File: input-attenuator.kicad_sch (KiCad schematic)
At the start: 44 parts, among them J1 DC_INTF, J2 RF_IN, J3 RX_1_RF, J4 RX_2_RF, K1 EE2-5TNU-L, K2 EE2-5TNU-L, K3 EE2-5TNU-L, K4 EE2-5TNU-L, Q1 MMBT3904, Q2 MMBT3904, Q3 MMBT3904, Q4 MMBT3904, Q5 MMBT3904, Q6 MMBT3904, Q7 MMBT3904, Q8 MMBT3904, U1 74HC595

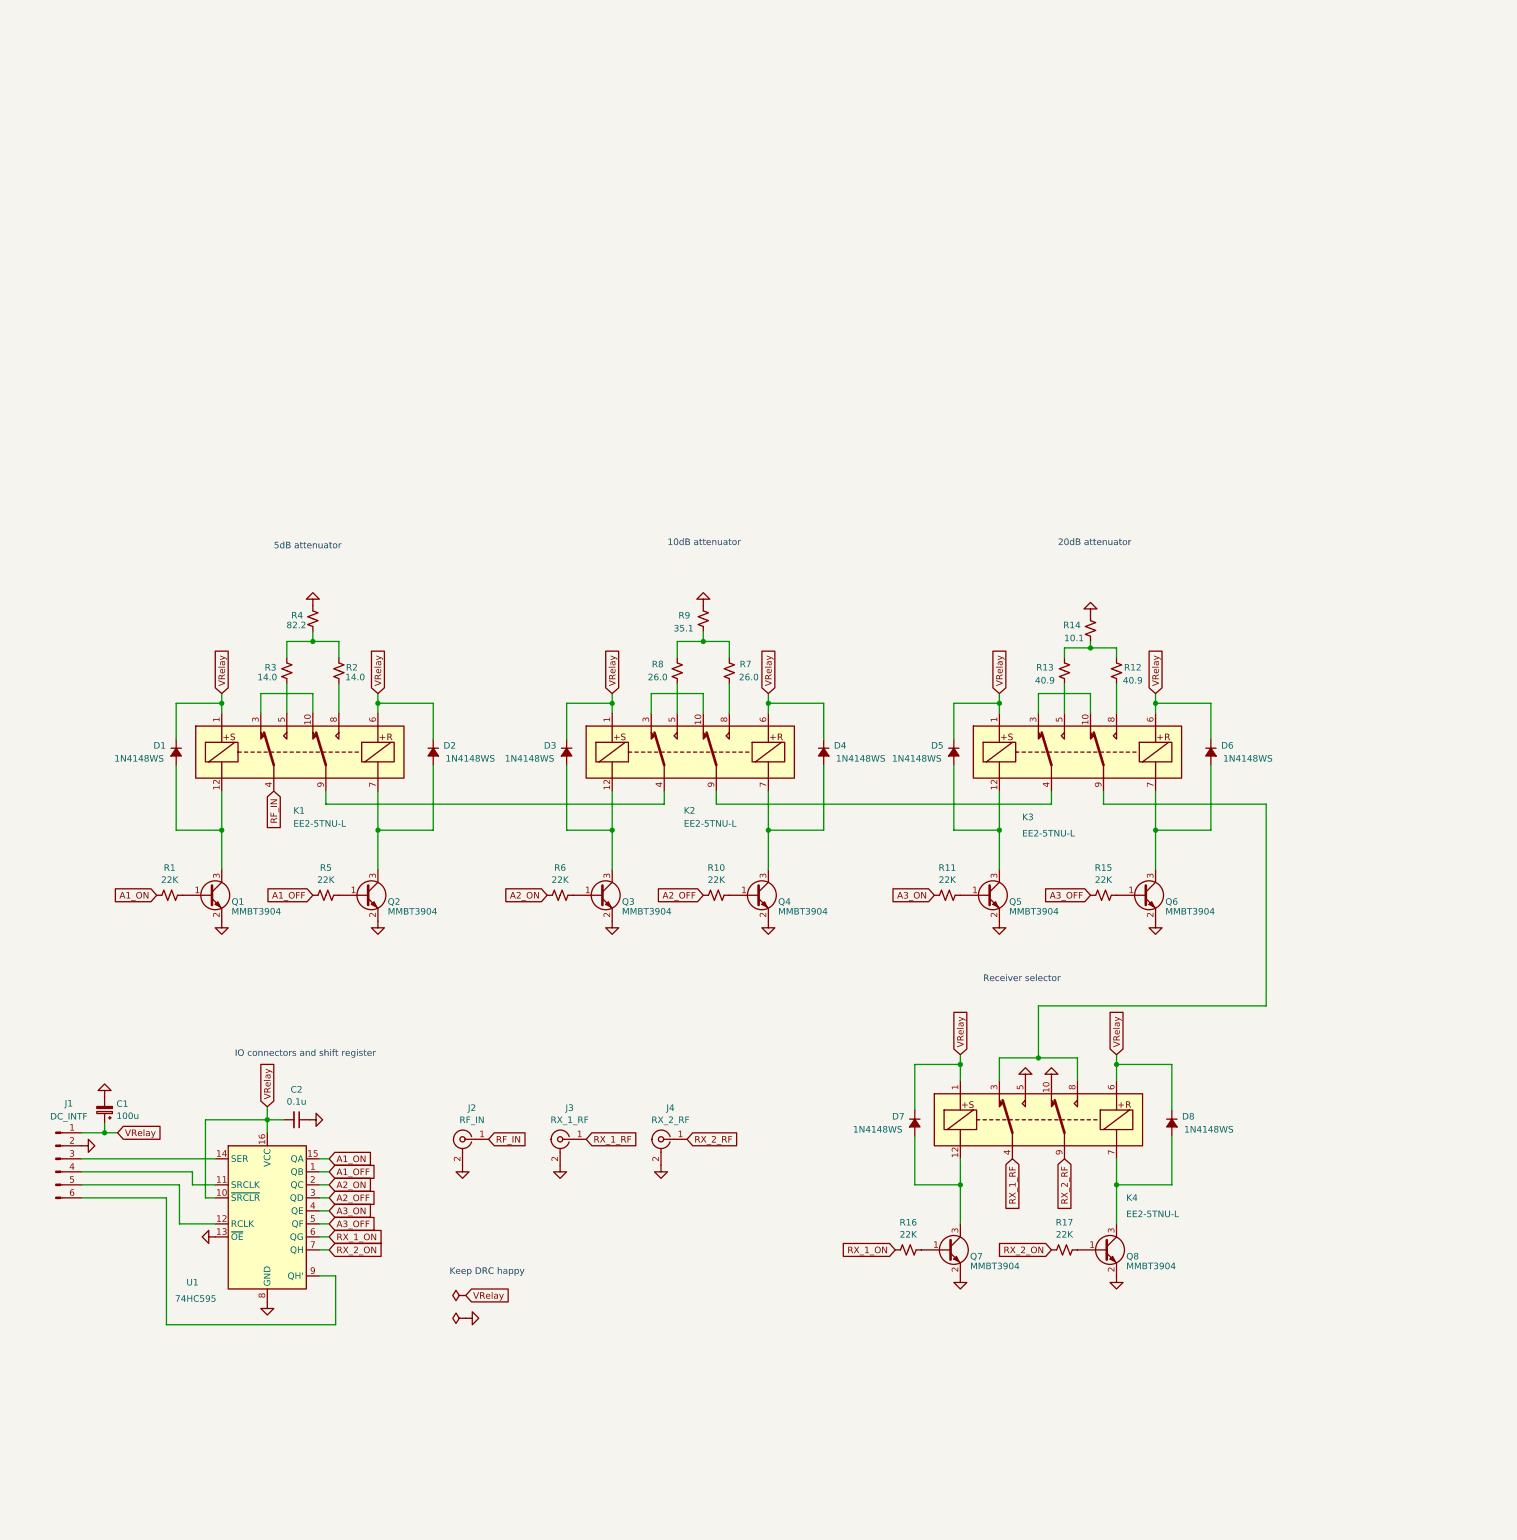
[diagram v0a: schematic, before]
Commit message: noComment
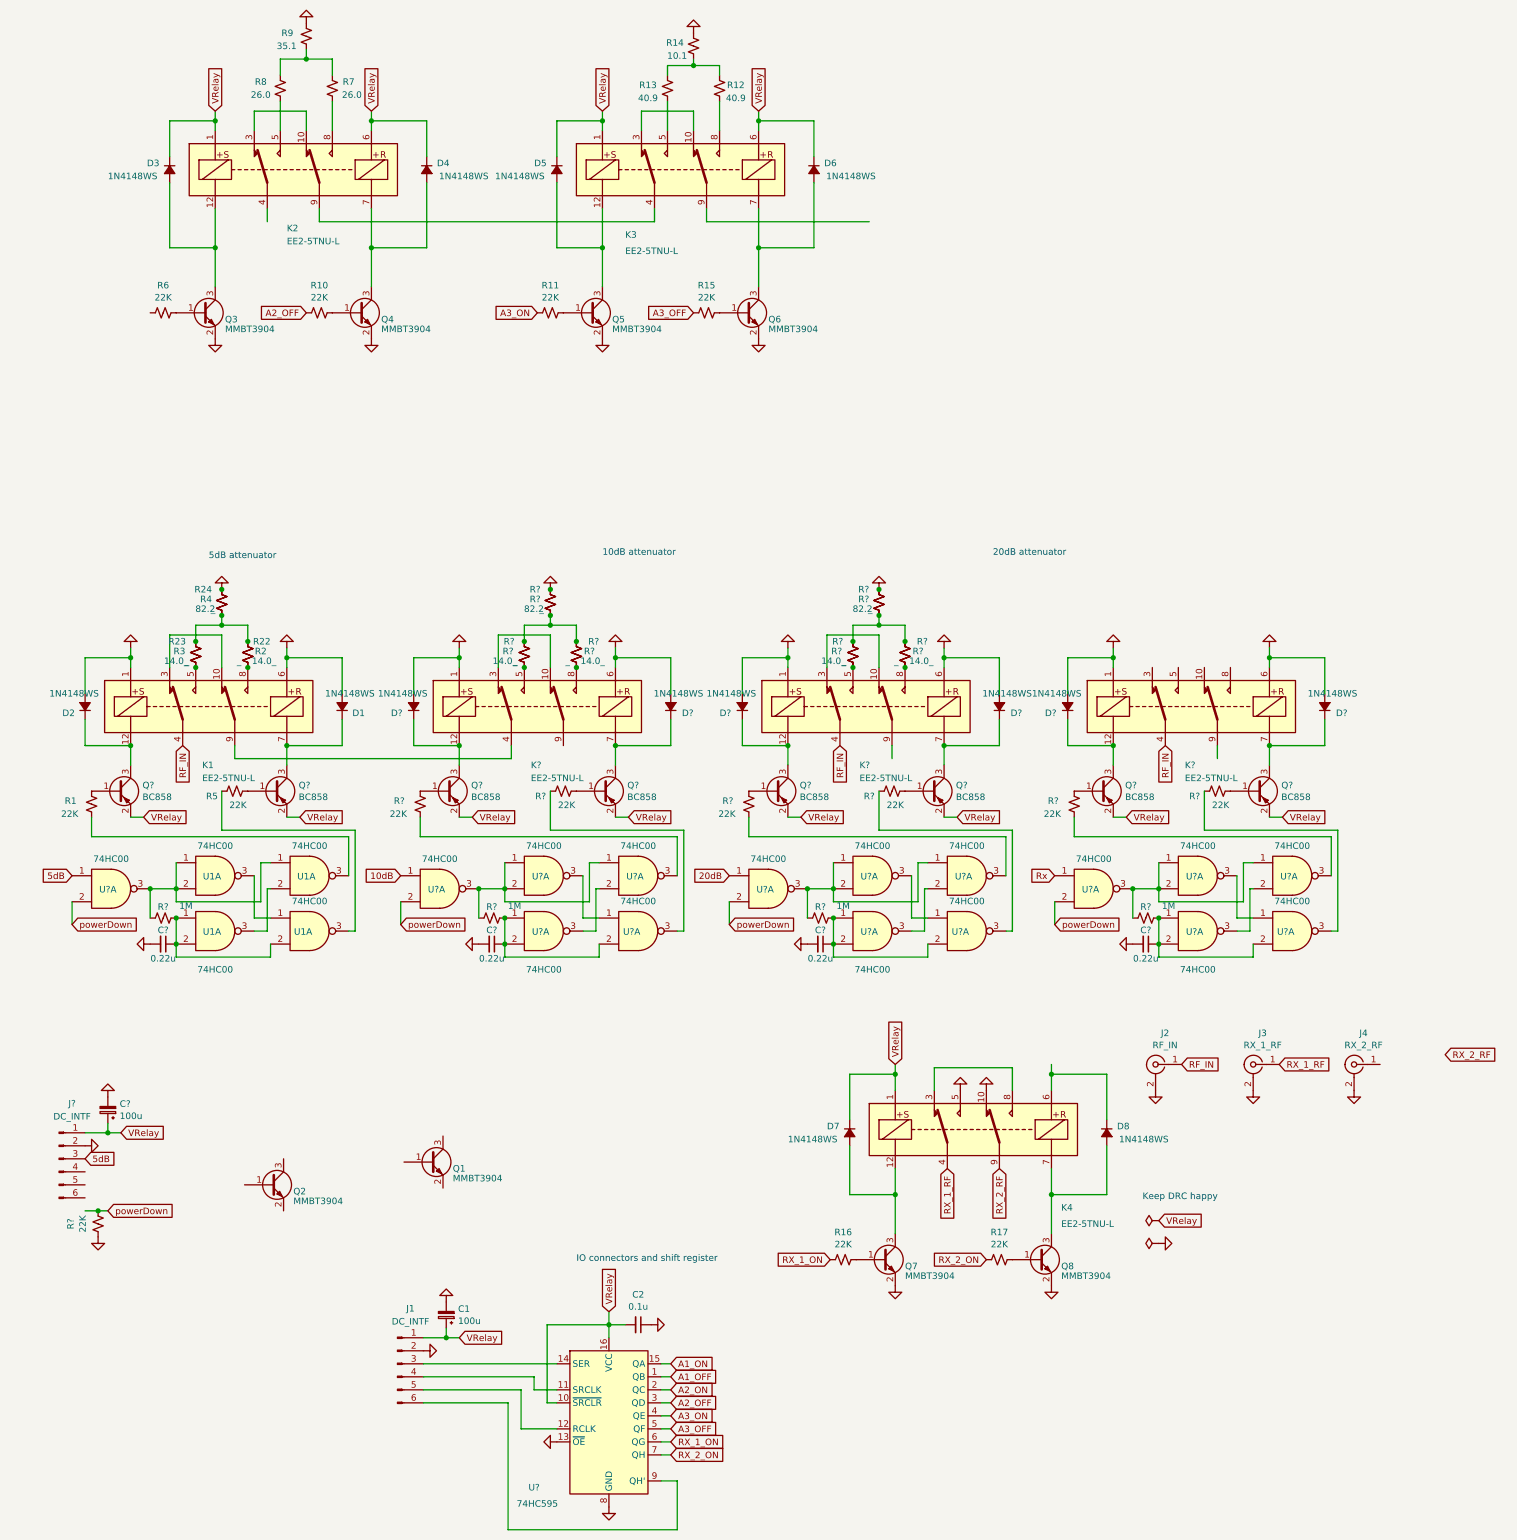
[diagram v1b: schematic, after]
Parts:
- added C? (x4): 0.22u, Capacitor_SMD:C_0805_2012Metric, symbol Device:C_Small
- added C?: 100u, Capacitor_SMD:CP_Elec_6.3x5.4_Nichicon, symbol Device:CP_Small
- added D? (x6): 1N4148WS, Diode_SMD:D_SOD-323, symbol Device:D_Small_ALT
- added J?: DC_INTF, Connector_PinHeader_2.54mm:PinHeader_1x06_P2.54mm_Vertical, symbol Connector:Conn_01x06_Male
- added K? (x3): EE2-5TNU-L, Relay_SMD:Relay_DPDT_Kemet_EE2_NU_DoubleCoil, symbol Relay:EE2-5TNU
- added Q? (x8): BC858, Package_TO_SOT_SMD:SOT-23, symbol Transistor_BJT:BC858
- added R22, R23, R24, R? (x6): _, Resistor_SMD:R_0805_2012Metric, symbol Device:R_Small_US
- added R? (x7): 22K, Resistor_SMD:R_0805_2012Metric, symbol Device:R_Small_US
- added R? (x4): 1M, Resistor_SMD:R_0805_2012Metric, symbol Device:R_Small_US
- added R? (x2): 82.2, Resistor_SMD:R_0805_2012Metric, symbol Device:R_Small_US
- added R? (x4): 14.0_, Resistor_SMD:R_0805_2012Metric, symbol Device:R_Small_US
- added U1 (x4), U? (x16): 74HC00, symbol 74xx:74HC00
- R2, R3: value 14.0 -> 14.0_
- R4: value 82.2 -> 82.2
- renumbered U1 to U?
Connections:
- net A1_OFF: no longer R5.1
- net A1_ON: no longer R1.1
- net A2_ON: no longer R6.1
- net GND: now also D1.2 (A), D2.2 (A), K1.1, K1.6, C?.2, C?.2, C?.2, C?.2, C?.2, D?.2 (A), D?.2 (A), D?.2 (A), D?.2 (A), D?.2 (A), D?.2 (A), J?.2 (Pin_2), K?.1, K?.1, K?.1, K?.6, K?.6, K?.6, R24.2, R?.1, R?.2, R?.2, R?.2, R?.2; no longer Q1.2 (E), Q2.2 (E)
- net RF_IN: now also K?.4, K?.4
- net RX_2_RF: no longer J4.1 (In)
- net VRelay: now also C?.1, J?.1 (Pin_1), Q?.2 (E), Q?.2 (E), Q?.2 (E), Q?.2 (E), Q?.2 (E), Q?.2 (E), Q?.2 (E), Q?.2 (E); no longer D1.1 (K), D2.1 (K), D8.1 (K), K1.1, K1.6, K4.6
- net at K1.5, R3.1: now also R23.1
- net at K1.8, R2.2: now also R22.1
- net at K1.9: now also K?.4; no longer K2.4
- net at Q1.1 (B): no longer R1.2
- net at R5.2: now also Q?.1 (B); no longer Q2.1 (B)
- net at R2.1, R3.2, R4.1: now also R22.2, R23.2, R24.1
- net at K4.3, K4.8: no longer K3.9
- new net: D2.1 (K), K1.12, Q?.3 (C)
- new net: D1.1 (K), K1.7, Q?.3 (C)
- new net: R1.1, U1.3
- new net: Q?.1 (B), R1.2
- new net: R5.1, U1.3
- new net: D8.1 (K), K4.6
- new net: R?.1, U?.3 (x6)
- new net: Q?.1 (B), R?.2 (x6)
- new net: D?.1 (K), K?.7, Q?.3 (C) (x3)
- new net: R?.1, U1.1, U1.1, U1.2, U?.3
- new net: U1.1, U1.3
- new net: C?.1, R?.2, U1.1, U1.2, U1.2
- new net: U?.1, U?.3 (x3)
- new net: C?.1, R?.2, U?.1, U?.2, U?.2 (x3)
- new net: R?.1, U?.1, U?.1, U?.2, U?.3 (x3)
- new net: U?.2, U?.3 (x3)
- new net: K?.5, R?.1, R?.1 (x2)
- new net: R?.1, R?.1, R?.1, R?.2, R?.2, R?.2 (x2)
- new net: D?.1 (K), K?.12, Q?.3 (C) (x3)
- new net: U1.2, U1.3
- new net: K?.10, K?.3 (x2)
- new net: K?.8, R?.1, R?.2 (x2)
- new net 10dB: U?.1
- new net 20dB: U?.1
- new net 5dB: J?.3 (Pin_3), U?.1
- new net Rx: U?.1
- new net powerDown: R?.2, U?.2, U?.2, U?.2, U?.2
- now unconnected: Q1.3 (C), Q2.3 (C)
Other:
- note removed: "Receiver selector"
- moved on the sheet: C1, C2, D1, D2, D3, D4, D5, D6, D7, D8, J1, J2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

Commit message: relays
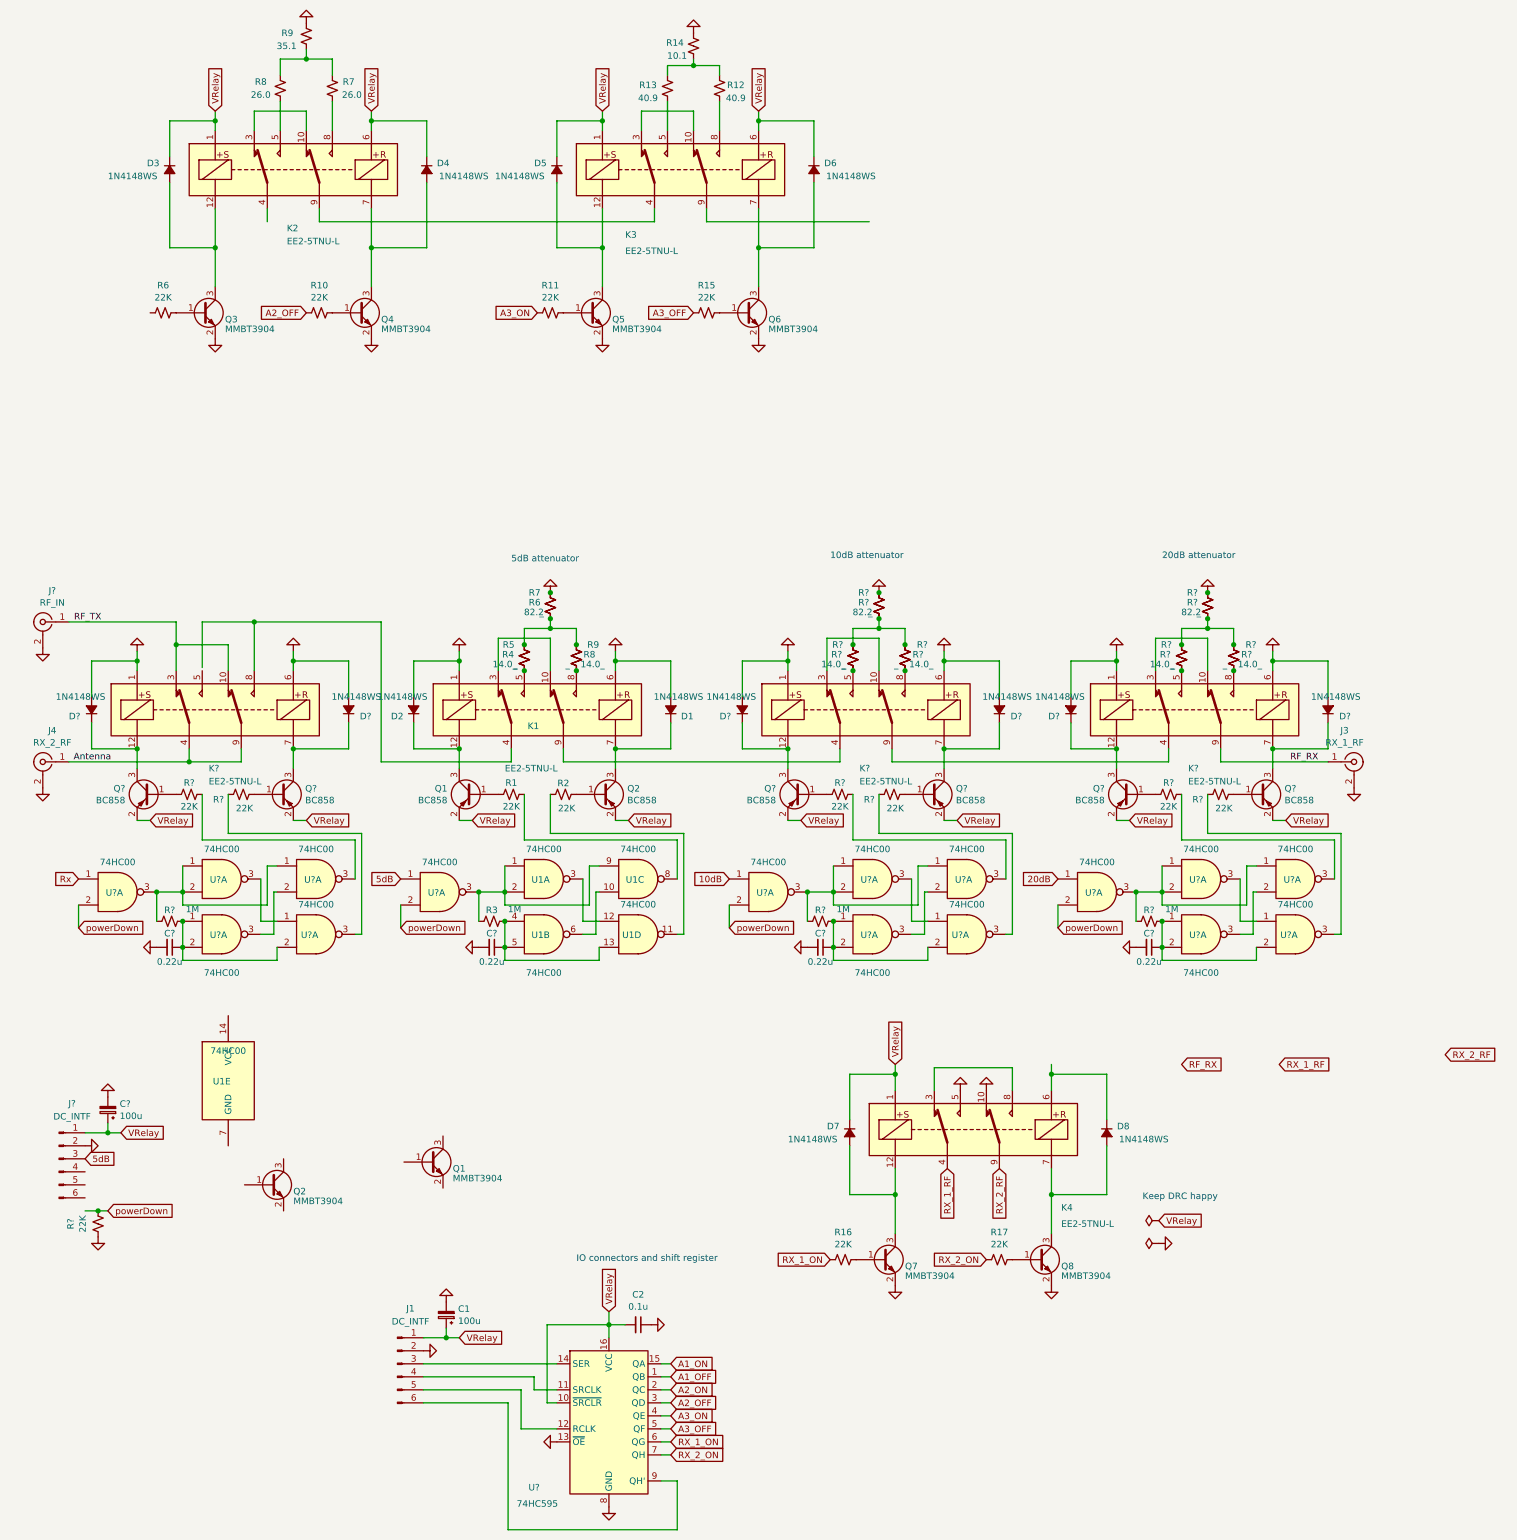
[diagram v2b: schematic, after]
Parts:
- removed J2: RF_IN, Connector_Coaxial:SMA_Amphenol_132134_Vertical, symbol Connector:Conn_Coaxial
- removed Q? (x3): BC858, Package_TO_SOT_SMD:SOT-23, symbol Transistor_BJT:BC858
- removed R? (x3): 22K, Resistor_SMD:R_0805_2012Metric, symbol Device:R_Small_US
- added J?: RF_IN, Connector_Coaxial:SMA_Amphenol_132134_Vertical, symbol Connector:Conn_Coaxial
- added Q? (x3): BC858, Package_TO_SOT_SMD:SOT-23, symbol Transistor_BJT:BC858
- added R? (x3): 22K, Resistor_SMD:R_0805_2012Metric, symbol Device:R_Small_US
- added unit 5 of U1
- gave numbers to parts that had none: 3
- renumbered R5 to R2, R3 to R4, R23 to R5, R4 to R6, R24 to R7, R2 to R8, R22 to R9
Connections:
- net GND: now also J?.2 (Ext)
- net RX_1_RF: no longer J3.1 (In)
- net VRelay: now also Q?.2 (E), Q?.2 (E), Q?.2 (E)
- net at R1.1: now also U1.8; no longer U1.3
- net at R2.1: now also U1.11; no longer U1.3
- net Antenna: now reaches J4.1 (In)
- net Antenna: now also K?.4, K?.9
- net at R3.1, U1.1, U1.2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: now also U1.9; no longer U1.1
- net at U1.3: now also U1.12; no longer U1.1
- net at U?.3: now also R?.1 (x3)
- net at D?.1 (K), K?.12: now also Q?.3 (C) (x3)
- net RF_RX: now reaches K?.9
- net RF_RX: now also J3.1 (In)
- net RF_TX: now reaches K?.10
- net RF_TX: now also K?.3, J?.1 (In)
- net at K?.8: now also K1.4
- net at K?.9: now also K?.4
- removed net RF_IN: K1.4, K?.4, K?.4
- new net: C?.1, R3.2, U1.13, U1.4, U1.5
- new net: U1.10, U1.6
- new net: Q?.1 (B), R?.2 (x3)
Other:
- moved on the sheet: C?, D1, D2, D?, J3, J4, K1, K?, Q1, Q2, Q?, R1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
